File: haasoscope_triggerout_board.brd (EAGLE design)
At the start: 31 x 22 mm, 6 parts, among them J1 2p-2.54, J2 2p-2.54

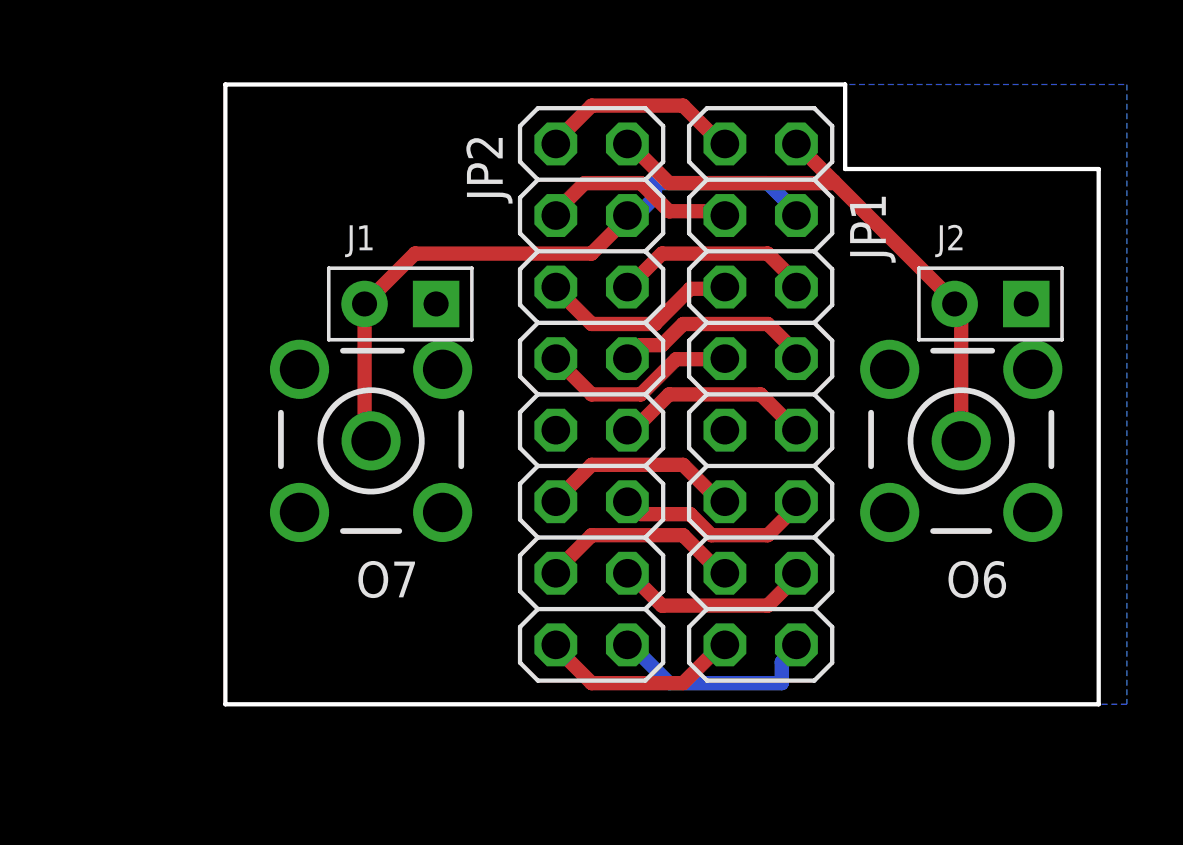
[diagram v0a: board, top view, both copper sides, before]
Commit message: trigout board
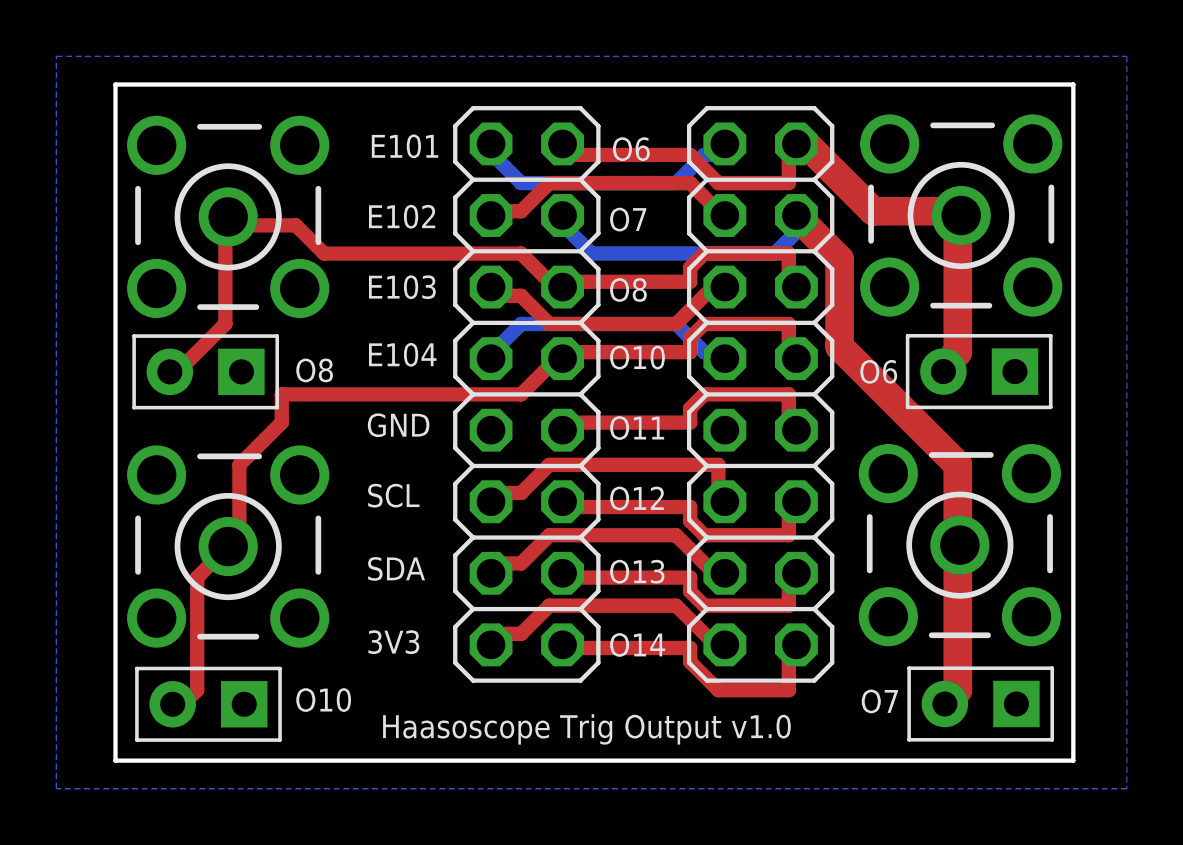
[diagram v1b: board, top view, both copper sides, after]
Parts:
- added J3, J4: 2p-2.54, Seeed-Connector:H2-2.54
- added O10, O8: BU-SMB-V, con-coax:BU-SMB-V
- moved J1 25.0 mm to (25.8, -0.99)
- moved O7 21.2 mm to (25.1, 4.65)
- moved O6 8.00 mm to (25.1, 16.4)
- moved J2 2.43 mm to (25.8, 10.8)
- moved JP2 2.30 mm to (9.70, 10.0)
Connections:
- net A10: now also J4.2, O10.1
- net A8: now also J3.2, O8.1
- net GND: now also J3.1, J4.1, O10.2, O10.3, O10.4, O10.5, O8.2, O8.3, O8.4, O8.5
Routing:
- net A10: track 7.13 -> 33.6 mm
- net A8: track 7.07 -> 29.5 mm
- net A7: track 23.0 -> 30.0 mm
- net A11: track 7.04 -> 10.4 mm
- net A14: track 7.59 -> 10.8 mm
- net A13: track 7.00 -> 10.2 mm
- net A12: track 7.07 -> 10.2 mm
- net SCL: track 7.09 -> 10.1 mm
- net E103: track 7.09 -> 9.65 mm
- net 3V3: track 7.15 -> 9.69 mm
- net SDA: track 7.14 -> 9.67 mm
- net E101: track 7.15 -> 9.68 mm
- net E104: track 7.04 -> 9.39 mm
- net E102: track 7.00 -> 9.27 mm
- net A6: track 20.9 -> 23.0 mm
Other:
- board size 31 x 22 mm -> 34 x 24 mm
- board text added: "3V3"
- board text added: "E101"
- board text added: "E102"
- board text added: "E103"
- board text added: "E104"
- board text added: "GND"
- board text added: "Haasoscope Trig Output v1.0"
- board text added: "O10"
- board text added: "O11"
- board text added: "O12"
- board text added: "O13"
- board text added: "O14"
- board text added: "O6"
- board text added: "O7"
- board text added: "O8"
- board text added: "SCL"
- board text added: "SDA"
